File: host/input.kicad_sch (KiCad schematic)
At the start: 22 parts, among them J2 Conn_01x04, J24 Conn_01x06, J4 Conn_01x06, U1 PCA9615DP

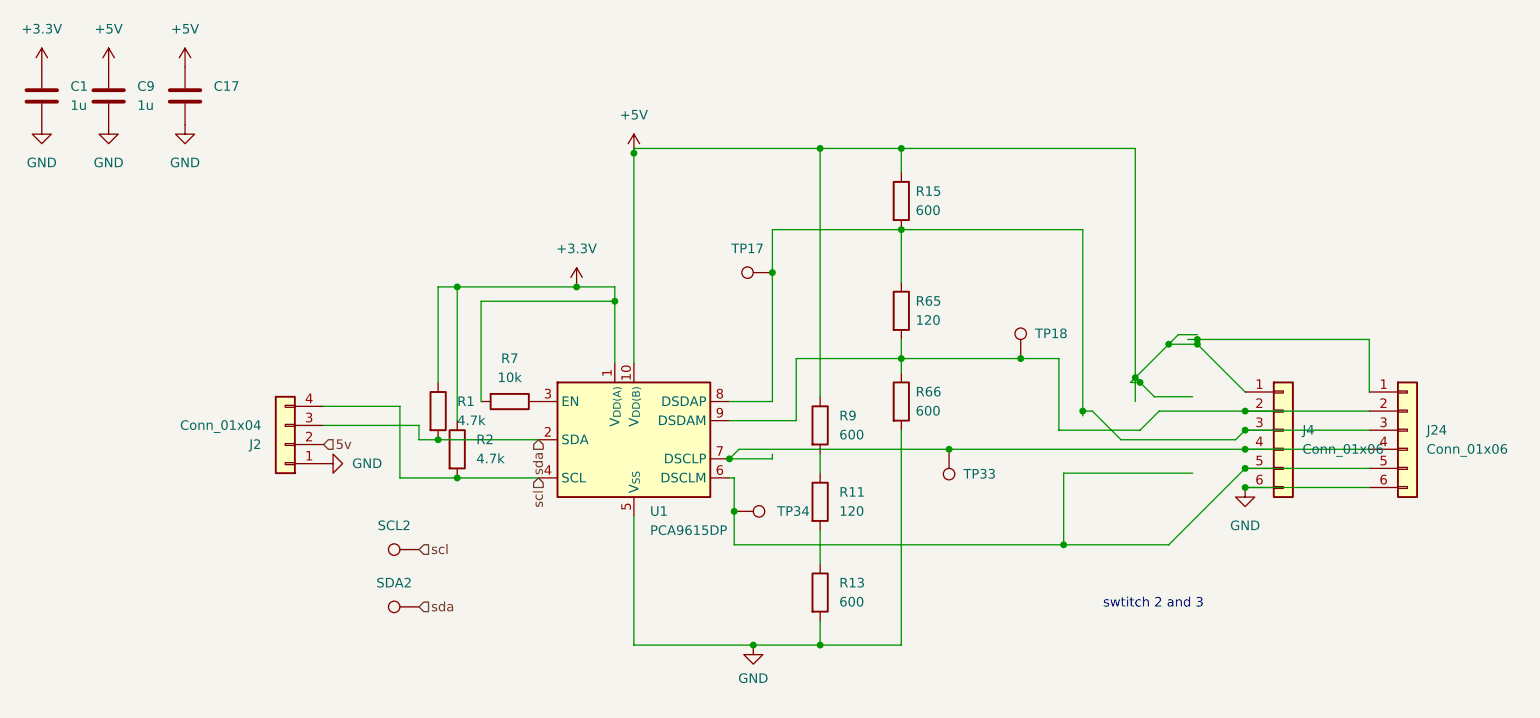
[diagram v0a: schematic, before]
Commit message: started host board layout v2
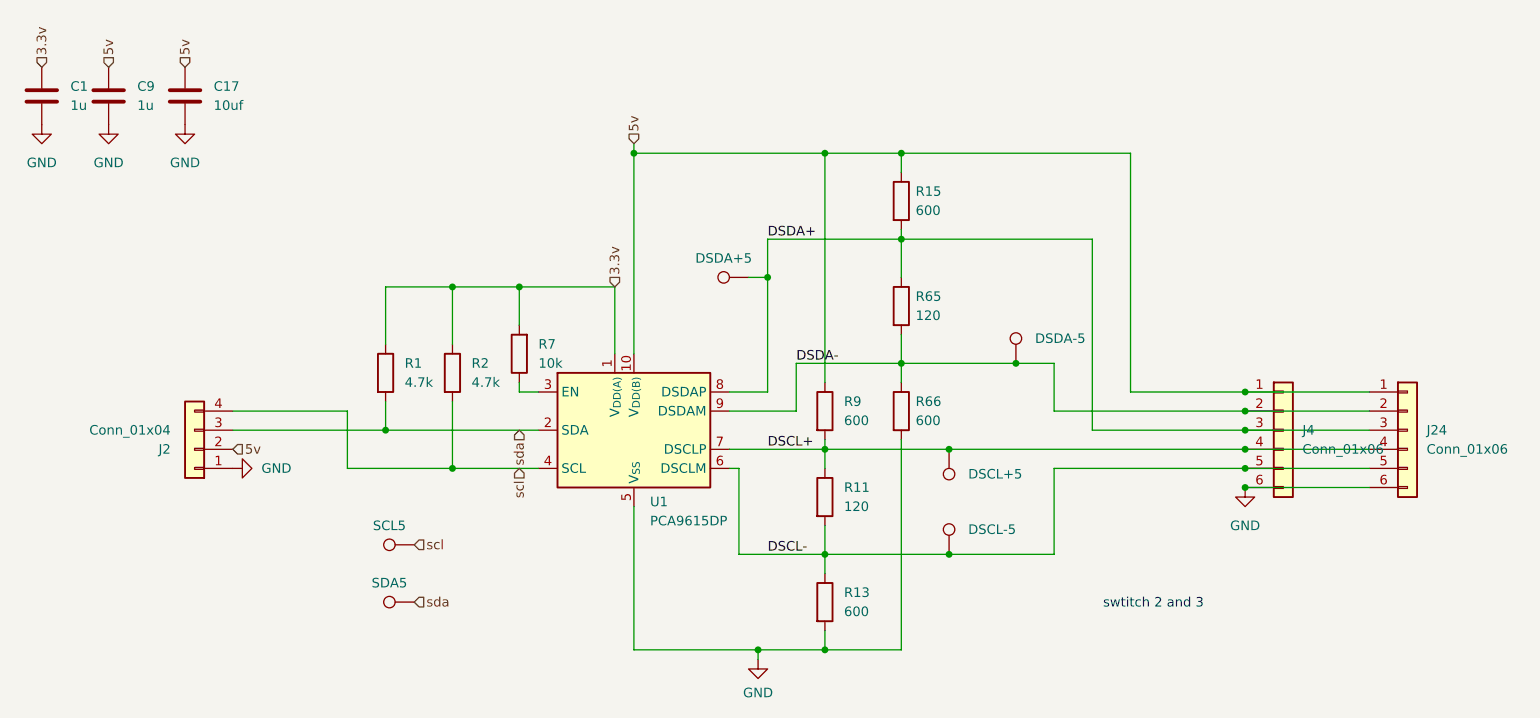
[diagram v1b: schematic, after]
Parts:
- renumbered TP33 to DSCL+5, TP34 to DSCL-5, TP17 to DSDA+5, TP18 to DSDA-5, SCL2 to SCL5, SDA2 to SDA5
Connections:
- net +5V is gone; now on net 5v: C17.1, C9.1, J24.1 (Pin_1), J4.1 (Pin_1), R15.1, R9.1, U1.10 (V_{DD(B)})
- net DSCL-: now reaches R11.2, R13.1
- net DSCL-: now also DSCL-5.1, J24.5 (Pin_5), J4.5 (Pin_5), U1.6 (DSCLM)
- net DSCL+: now reaches R11.1, R9.2
- net DSCL+: now also DSCL+5.1, J24.4 (Pin_4), J4.4 (Pin_4), U1.7 (DSCLP)
- net DSDA-: now reaches DSDA-5.1, J24.2 (Pin_2), J4.2 (Pin_2), R65.2, R66.1, U1.9 (DSDAM)
- net DSDA+: now reaches DSDA+5.1, J24.3 (Pin_3), J4.3 (Pin_3), R15.2, R65.1, U1.8 (DSDAP)
- net +3.3V renamed 3.3v
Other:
- moved on the sheet: DSCL-5, DSDA+5, DSDA-5, J2, R1, R11, R13, R2, R65, R66, R7, R9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
